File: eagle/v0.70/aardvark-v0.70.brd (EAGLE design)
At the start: 25.4 x 88.9 mm, 21 parts, among them IC1 LM1117-3.3, U1 CH340C, X1 MINI-USB-32005-201

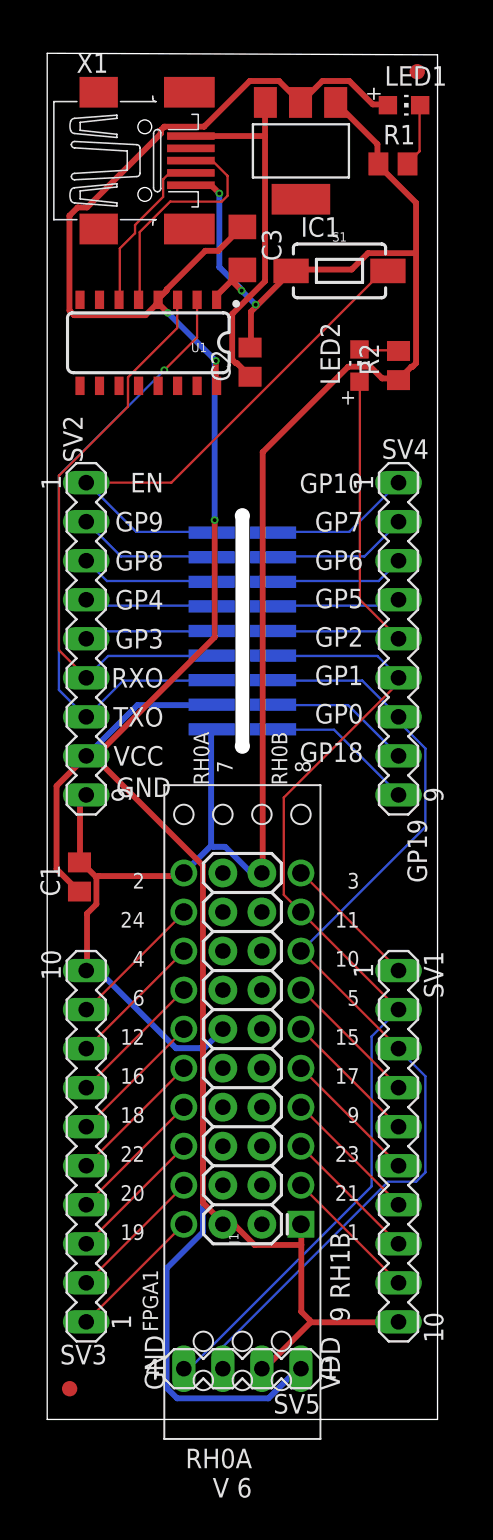
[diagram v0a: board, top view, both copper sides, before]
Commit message: 0.70 release candidate
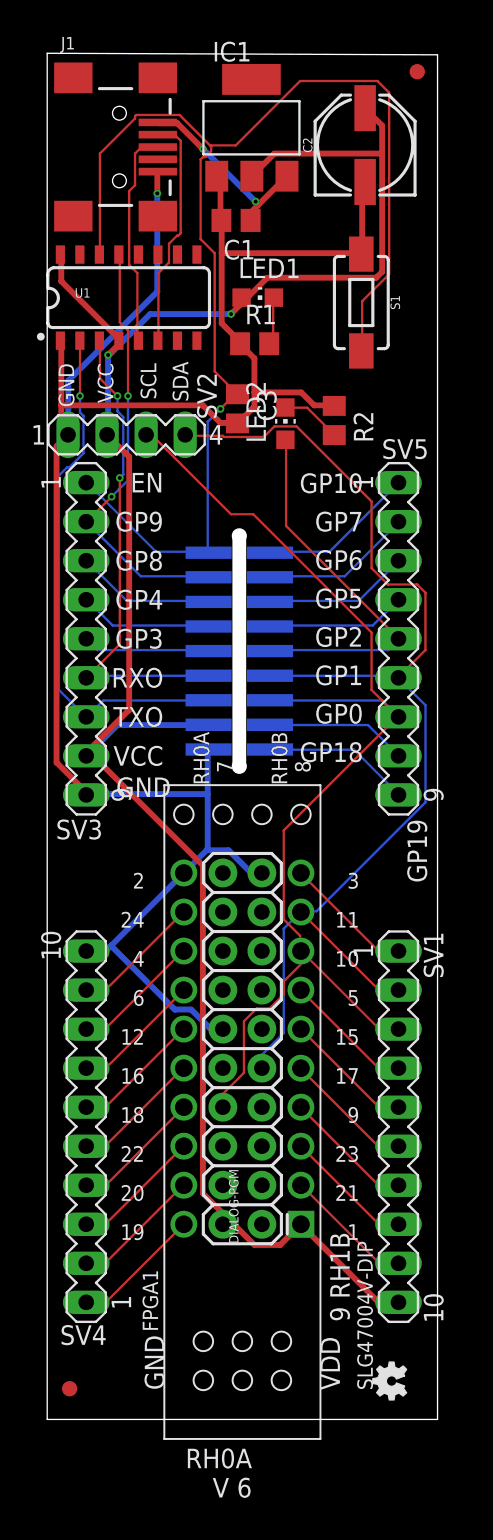
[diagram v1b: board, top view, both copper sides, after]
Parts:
- removed X1: MINI-USB-32005-201, con-cypressindustries:32005-201
- added DIALOG-PGM: (no value), SparkFun-Connectors:2X10
- added LOGO1: OSHW-LOGOMINI, SparkFun-Aesthetics:OSHW-LOGO-MINI
- C1: value 100nF -> 10uF
- C2: value 10uF -> 100uF; device rcl:C0805 -> SparkFun-Capacitors:PANASONIC_D
- C3: value (none) -> 4.7uF; device rcl:C1206 -> rcl:C0805
- FPGA1: value (none) -> SLG47004V-DIP
- J1: value (none) -> USB_MINI-B_SMT; device SparkFun-Connectors:2X10 -> SparkFun-Connectors:USB-MINIB
- LED1, LED2: device adafruit:CHIP-LED0805 -> led:CHIP-LED0805
- MOD1: value (none) -> ESP32-C3-M1; device aithinker-C3-M1:ESPRESSIF_ESP32-C3-01M -> aithinker-C3-M1:AITHINKER-C3-M1
- SV2: device con-lstb:MA09-1 -> con-lstb:MA04-1
- SV3: device con-lstb:MA10-1 -> con-lstb:MA09-1
- SV4: device con-lstb:MA09-1 -> con-lstb:MA10-1
- SV5: device con-lstb:MA04-1 -> con-lstb:MA09-1
- moved J1 70.7 mm to (4.70, 82.8), turned to 0 degrees
- moved SV5 48.6 mm to (22.9, 50.8), turned to 270 degrees
- moved C1 43.9 mm to (12.3, 78.0), turned to 180 degrees
- moved SV4 37.7 mm to (2.54, 19.1), turned to 90 degrees
- moved SV3 33.0 mm to (2.54, 50.8), turned to 270 degrees
- moved C2 16.0 mm to (20.7, 82.9)
- moved LED1 15.7 mm to (13.7, 73.0)
- moved R1 14.8 mm to (13.5, 70.0)
- moved SV2 13.5 mm to (5.17, 64.1), turned to 0 degrees
- moved C3 10.4 mm to (12.4, 65.8)
- moved LED2 6.13 mm to (15.5, 64.8)
- moved R2 5.50 mm to (18.7, 65.0), turned to 270 degrees
- moved IC1 3.55 mm to (13.3, 84.0), turned to 0 degrees
- moved U1 3.21 mm to (5.30, 73.0), turned to 0 degrees
- moved S1 2.50 mm to (20.4, 72.7), turned to 270 degrees
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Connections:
- removed net DTR: U1.13
- removed net RTS: U1.14
- removed net USBV: C2.1, IC1.3, X1.1
- new net VBUS: C1.1, IC1.3, J1.VBUS
- net EN: now also C3.1, SV3.1, U1.14; no longer SV2.1
- net GND: now also C2.-, DIALOG-PGM.12, DIALOG-PGM.19, J1.GND, SV2.1, SV3.9, SV4.10; no longer C2.2, J1.12, J1.19, SV2.9, SV3.10, SV5.1, X1.5
- net GP10: now also SV5.1; no longer SV4.1
- net GP18: now also SV5.8; no longer SV4.8
- net GP19: now also SV5.9; no longer SV4.9
- net GP2: now also SV5.5; no longer SV4.5
- net GP3: now also SV3.5; no longer SV2.5
- net GP4: now also SV3.4; no longer SV2.4
- net GP5: now also SV5.4; no longer SV4.4
- net GP6: now also SV5.3; no longer SV4.3
- net GP7: now also SV5.2; no longer SV4.2
- net GP8: now also SV3.3; no longer SV2.3
- net GP9: now also SV3.2, U1.13; no longer SV2.2
- net GPIO(PIN12): now also SV4.6; no longer SV3.6
- net GPIO(PIN16): now also SV4.5; no longer SV3.5
- net GPIO(PIN18): now also SV4.4; no longer SV3.4
- net GPIO(PIN19): now also SV4.1; no longer SV3.1
- net GPIO(PIN20): now also SV4.2; no longer SV3.2
- net OA0+(PIN4): now also SV4.8; no longer SV3.8
- net OA1-(PIN24): now also SV4.9; no longer SV3.9
- net OA1_OUT(PIN22): now also SV4.3; no longer SV3.3
- net RH0A(PIN6): now also SV4.7; no longer SV3.7
- net RXI: now also SV3.6; no longer SV2.6
- net SCL: now also DIALOG-PGM.8, SV2.3, SV5.7; no longer SV4.7, SV5.3
- net SDA: now also DIALOG-PGM.9, SV2.4, SV5.6; no longer SV4.6, SV5.4
- net TXO: now also SV3.7; no longer SV2.7
- net UD+: now also J1.D+; no longer X1.3
- net UD-: now also J1.D-; no longer X1.4
- net VCC: now also C2.+, DIALOG-PGM.2, SV2.2, SV3.8; no longer C1.1, C3.1, J1.2, SV2.8, SV5.2
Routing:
- net EN: track 34.9 -> 85.6 mm, vias 0 -> 1
- net GND: track 165.0 -> 138.2 mm, vias 3 -> 1
- net VCC: track 159.8 -> 134.7 mm, vias 3 -> 2
- net USBV: track 24.1 -> 0.00 mm
- net GP9: track 9.12 -> 28.2 mm, vias 0 -> 2
- net VBUS: track 0.00 -> 12.6 mm, vias 0 -> 2
- net SDA: track 65.9 -> 77.4 mm
- net SCL: track 65.6 -> 75.5 mm
- net TXO: track 40.8 -> 34.5 mm
- net RXI: track 37.3 -> 31.6 mm, vias 0 -> 2
- net UD-: track 11.0 -> 15.3 mm
- net GP2: track 26.2 -> 24.7 mm
- net N$1: track 2.62 -> 3.93 mm
- net N$3: track 4.16 -> 3.15 mm
- net UD+: track 15.2 -> 14.2 mm
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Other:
- board text added: "SCL"
- board text added: "SDA"
- board text added: "TriEmbed Community Aardvarck 0.70 CC BY-SA 2.0 ESP32-C3 + SLG47004V-DIP"
- board text removed: "TriEmbed Community Project Aardvarck 0.70 ESP32-C3 + SLG47004V-DIP"
